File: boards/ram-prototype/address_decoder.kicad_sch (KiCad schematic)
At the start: 33 parts, among them U1 74LVC1G04, U10 74LVC1G11, U11 74LVC1G11, U2 74LVC1G04, U3 74LVC1G04, U4 74LVC1G11, U5 74LVC1G11, U6 74LVC1G11, U7 74LVC1G11, U8 74LVC1G11, U9 74LVC1G11

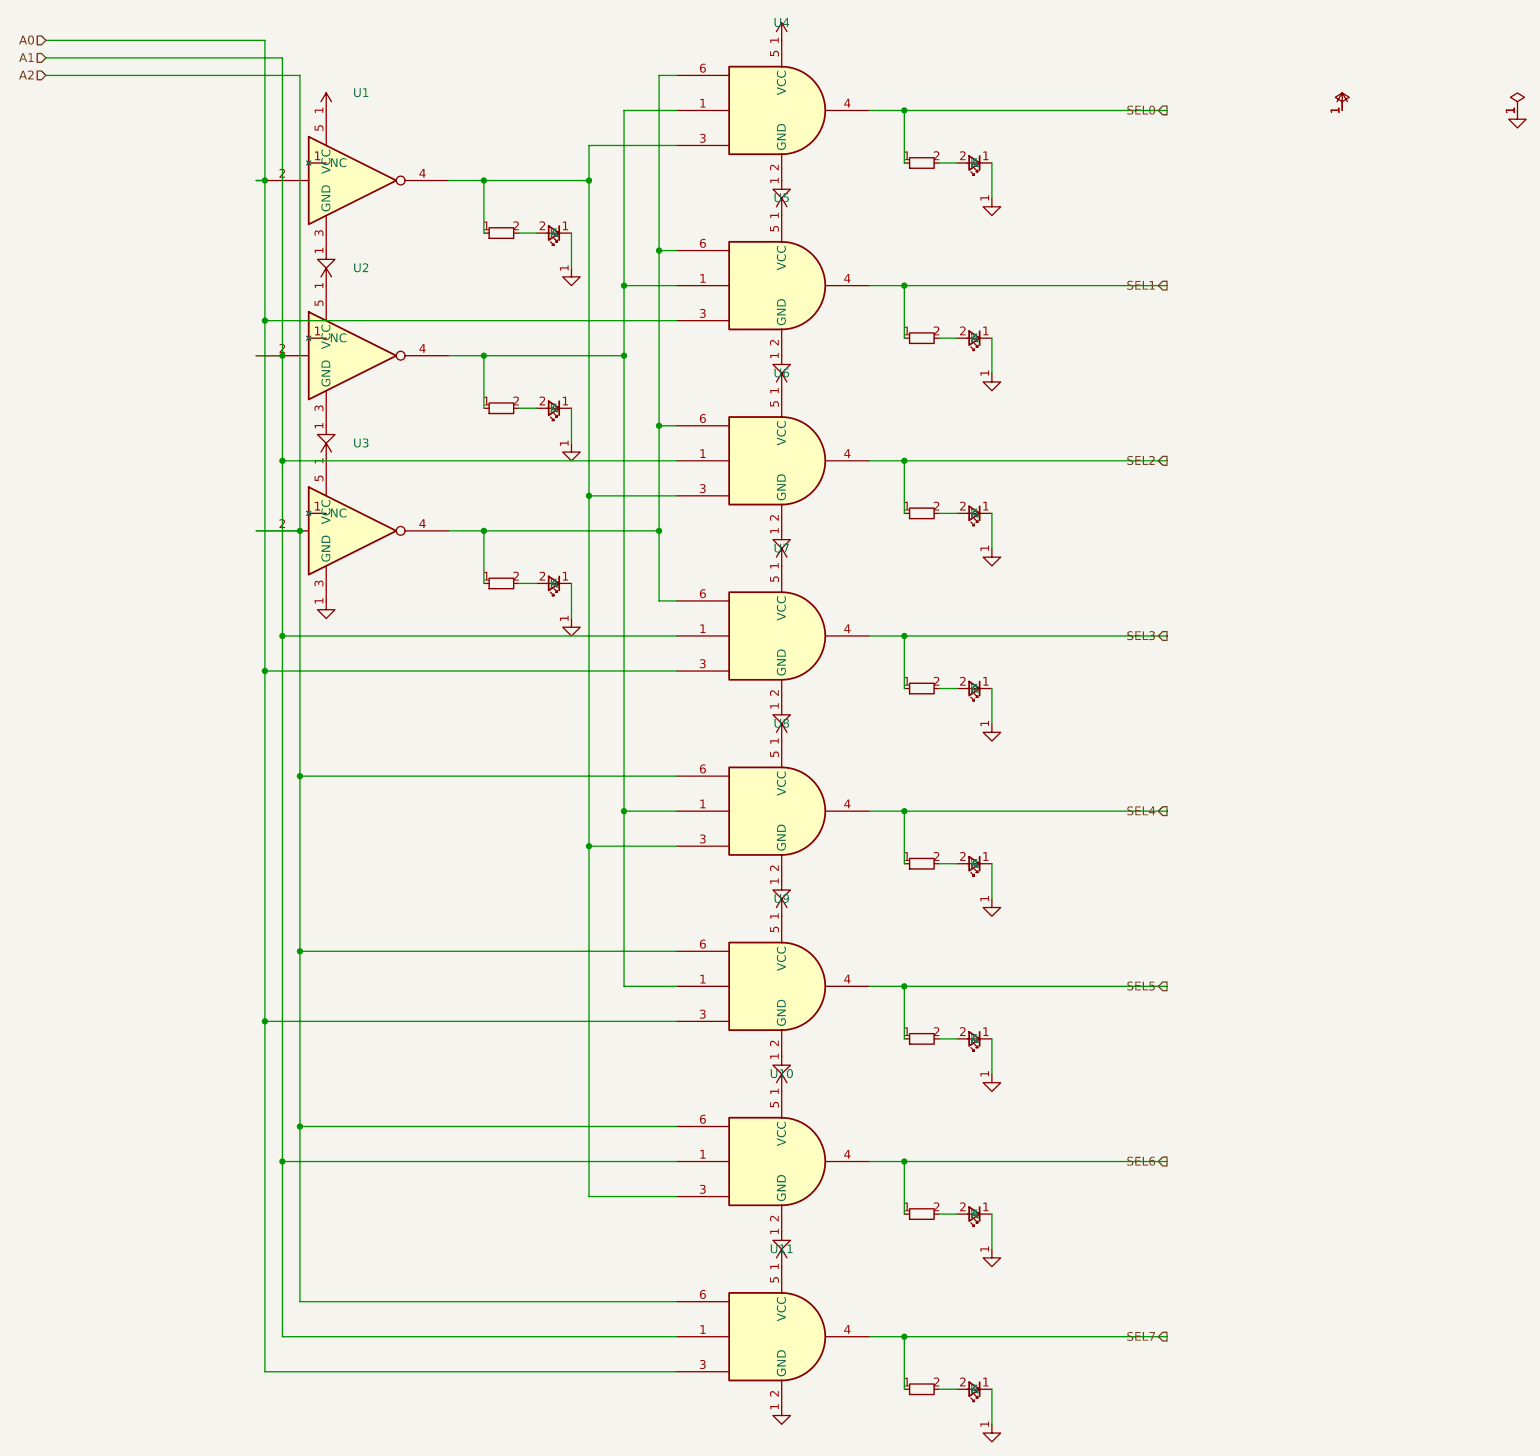
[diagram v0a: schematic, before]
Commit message: Fix a bunch of issues
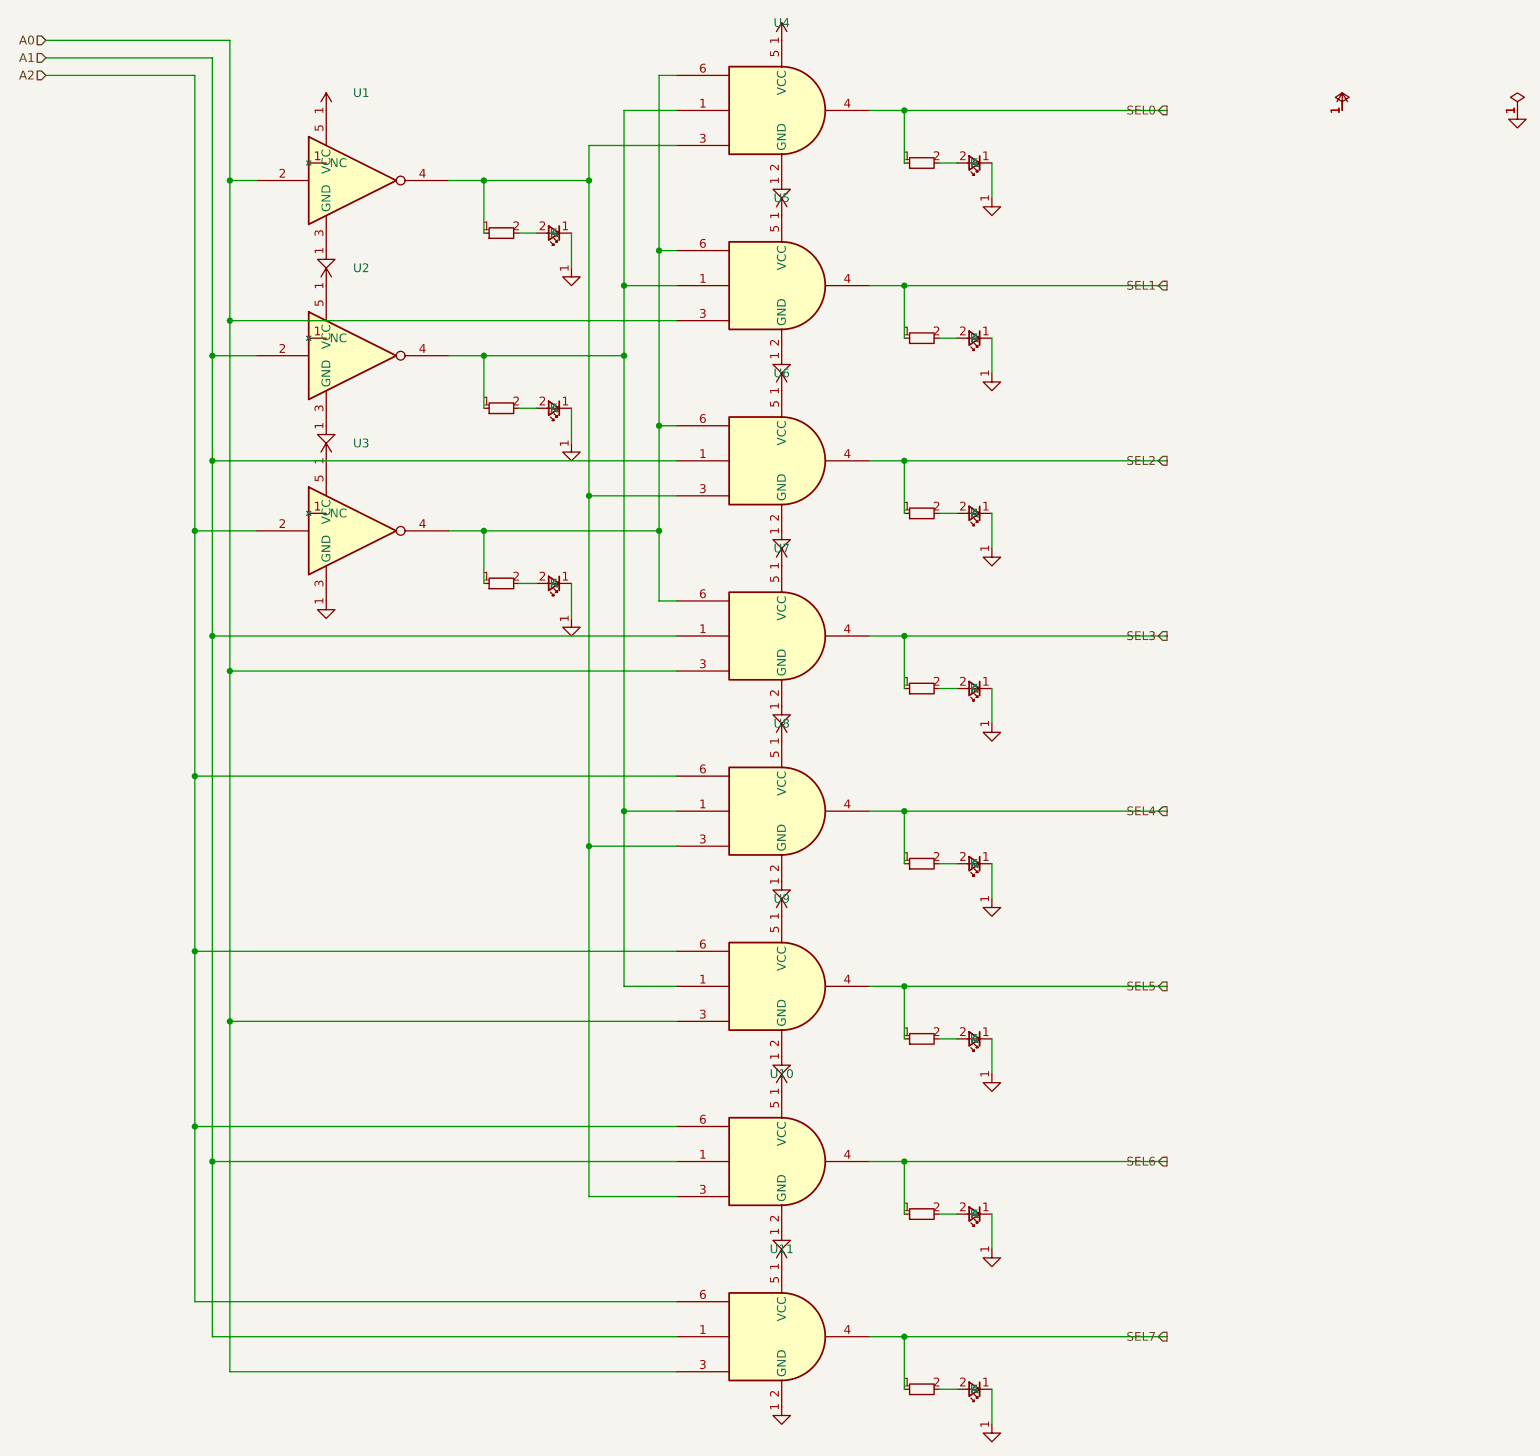
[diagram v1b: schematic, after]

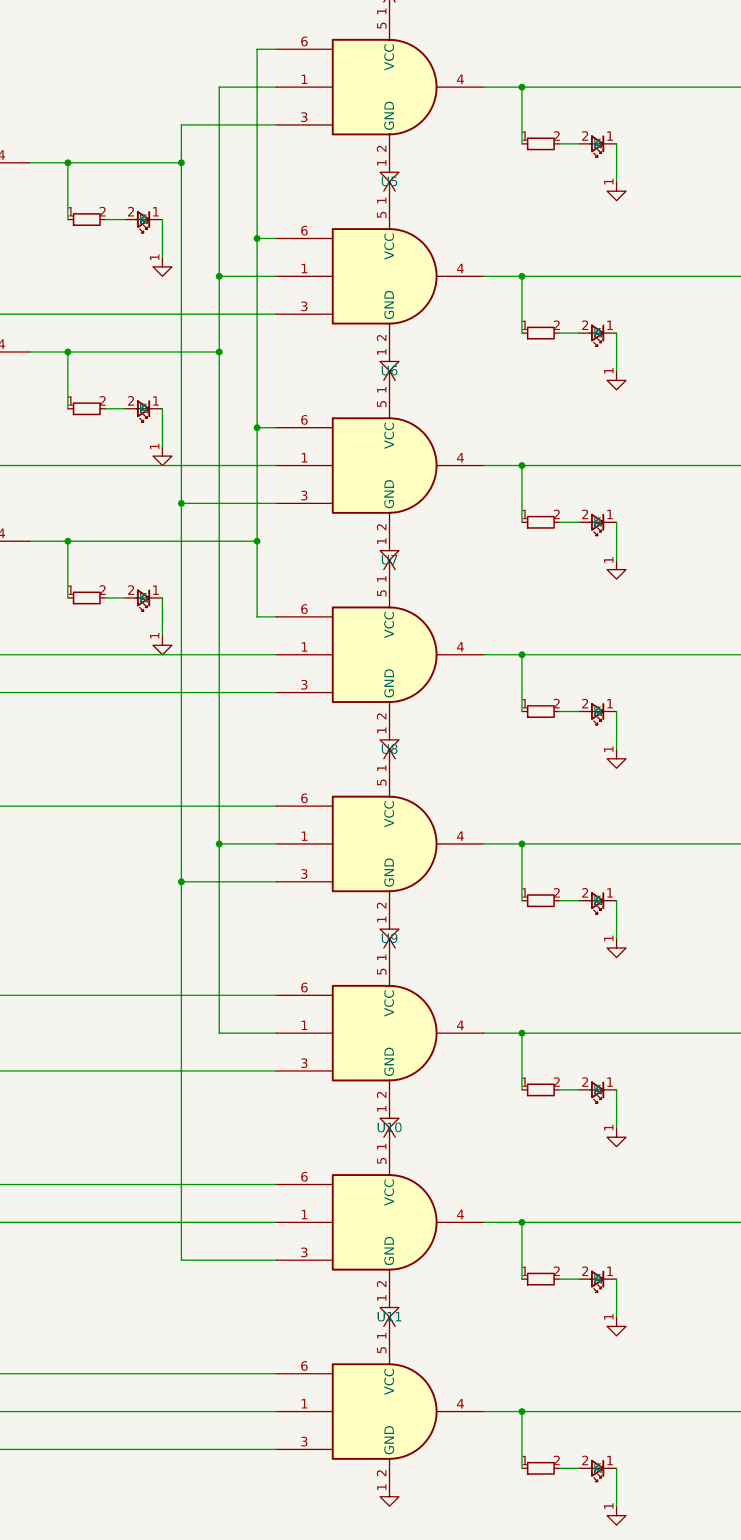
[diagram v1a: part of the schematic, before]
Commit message: Clean up root
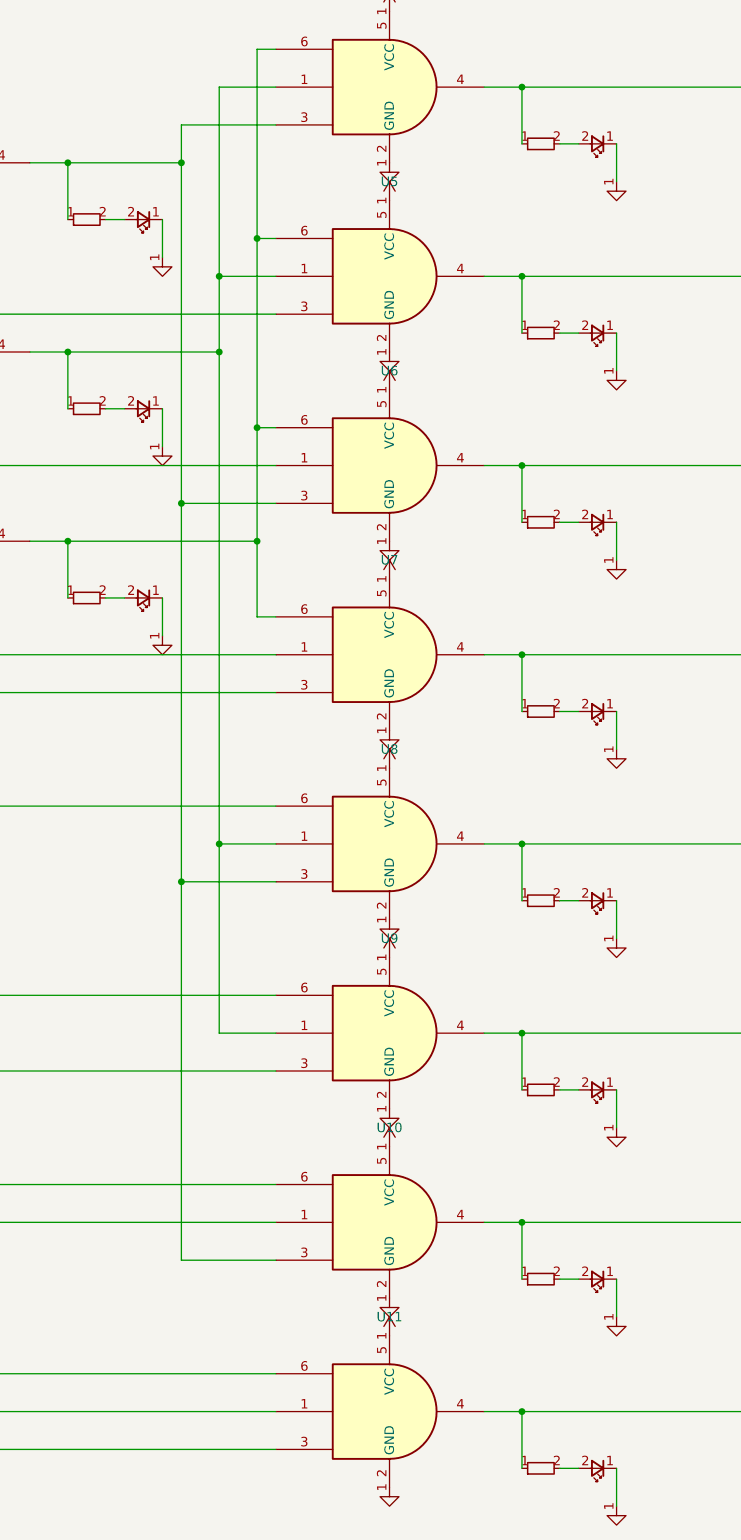
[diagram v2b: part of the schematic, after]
